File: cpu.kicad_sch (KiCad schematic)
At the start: 1 part

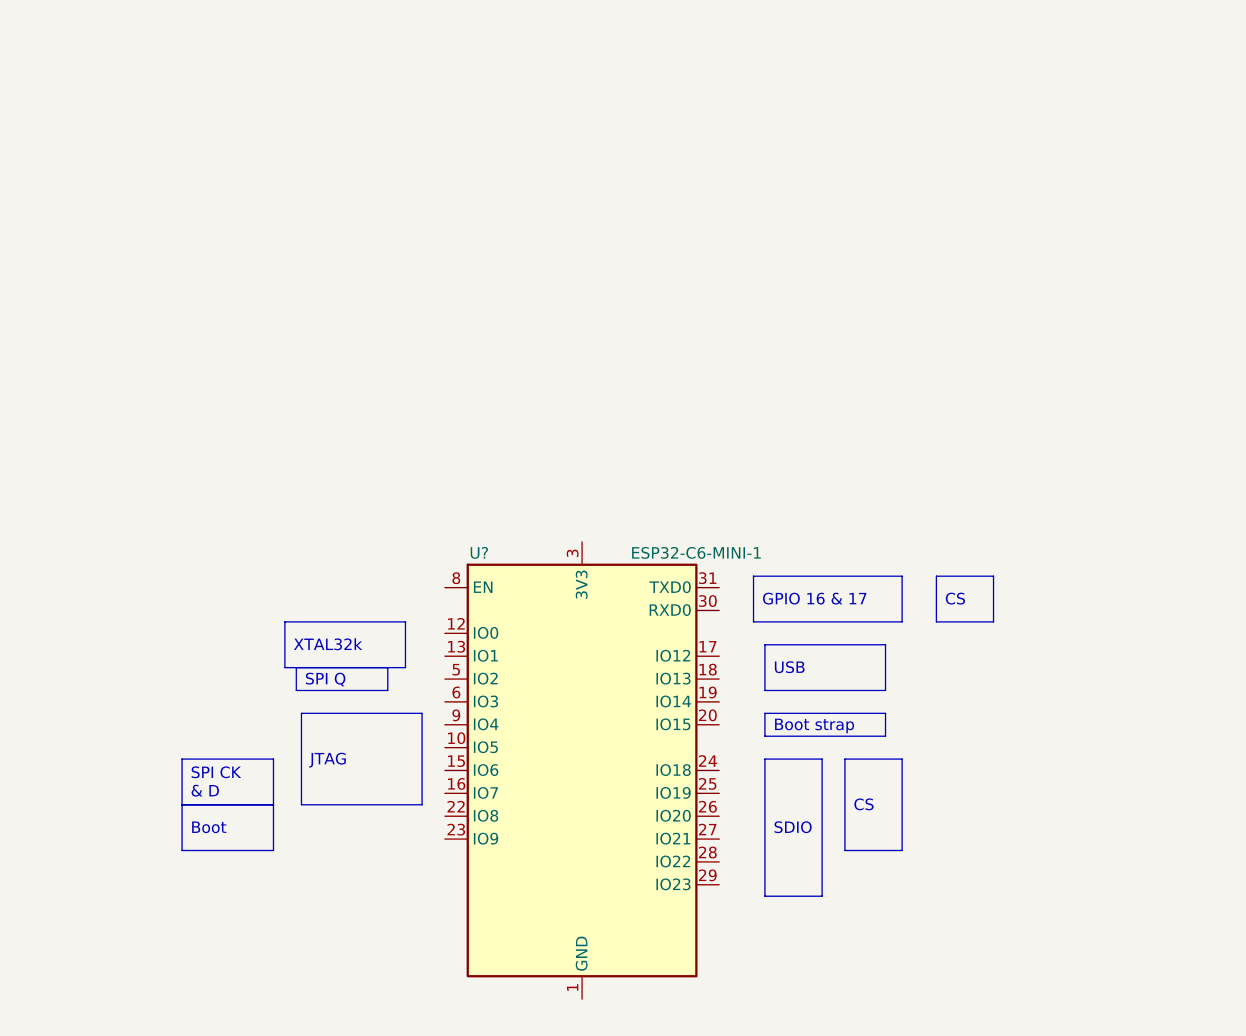
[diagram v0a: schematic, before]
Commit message: Schematic complete, maybe
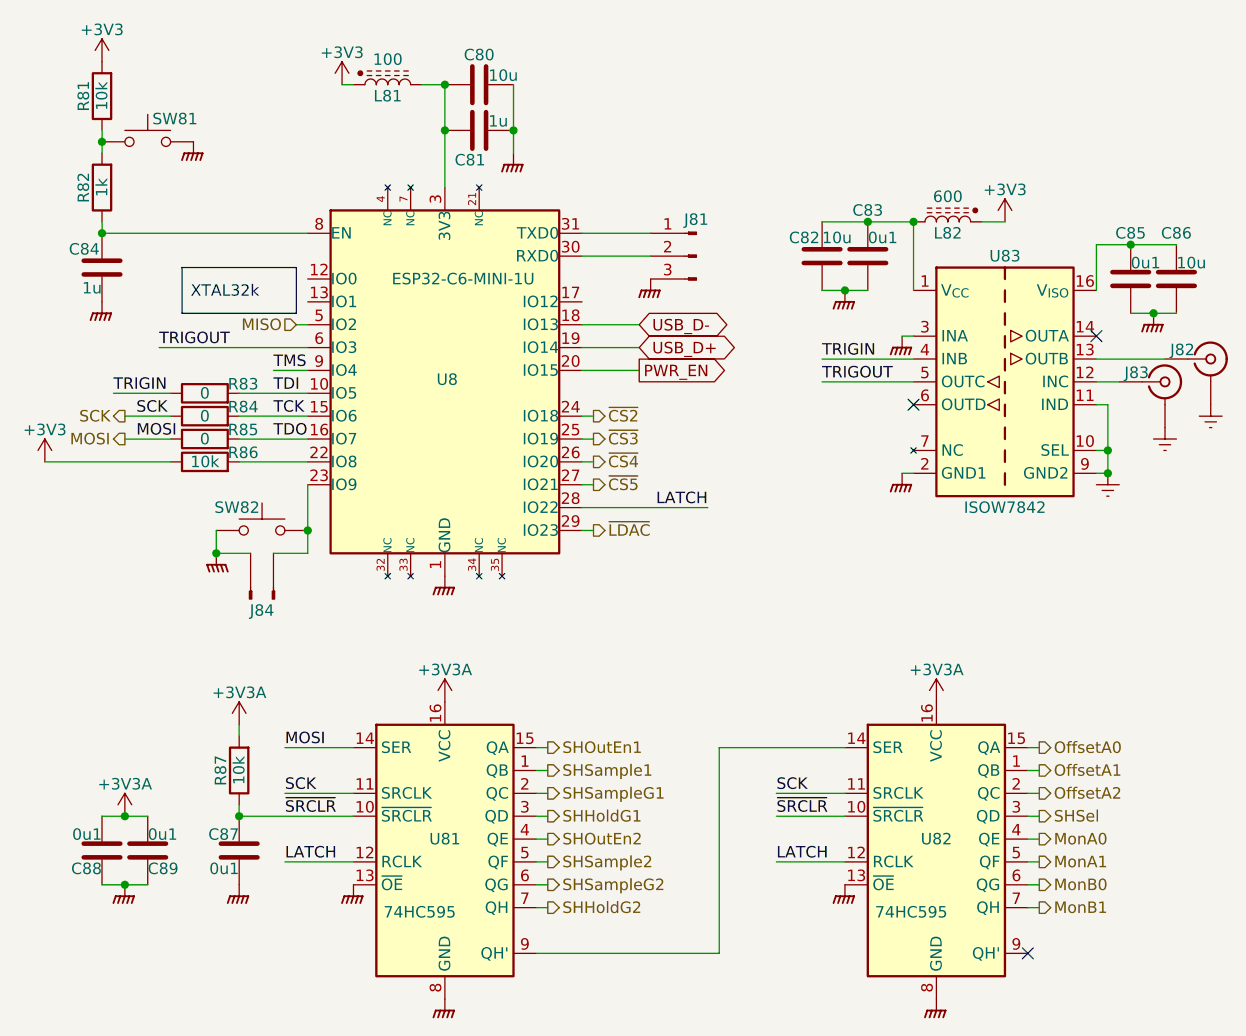
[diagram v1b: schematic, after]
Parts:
- removed U?: ESP32-C6-MINI-1, RF_Module:ESP32-C6-MINI-1, symbol RF_Module:ESP32-C6-MINI-1
- added C80, C82, C86: 10u, Capacitor_SMD:C_0603_1608Metric, symbol Device:C
- added C81, C84: 1u, Capacitor_SMD:C_0402_1005Metric, symbol Device:C
- added C83, C85, C87, C88, C89: 0u1, Capacitor_SMD:C_0402_1005Metric, symbol Device:C
- added J81: Conn_01x03_Pin, symbol Connector:Conn_01x03_Pin
- added J82, J83: Conn_Coaxial, symbol Connector:Conn_Coaxial
- added J84: Conn_01x02_Pin, symbol Connector:Conn_01x02_Pin
- added L81: 100, Inductor_SMD:L_0603_1608Metric, symbol Parts:L_Ferrite_Power
- added L82: 600, Inductor_SMD:L_0603_1608Metric, symbol Parts:L_Ferrite_Power
- added R81, R86, R87: 10k, Resistor_SMD:R_0402_1005Metric, symbol Device:R
- added R82: 1k, Resistor_SMD:R_0402_1005Metric, symbol Device:R
- added R83, R84, R85: 0, Resistor_SMD:R_0402_1005Metric, symbol Device:R
- added SW81, SW82: SW_Push, symbol Switch:SW_Push
- added U8: ESP32-C6-MINI-1U, RF_Module:ESP32-C6-MINI-1, symbol Parts:ESP32-C6-MINI-1U
- added U81, U82: 74HC595, Package_SO:SOIC-16_3.9x9.9mm_P1.27mm, symbol 74xx:74HC595
- added U83: ISOW7842, Package_SO:SOIC-16W_7.5x10.3mm_P1.27mm, symbol Parts:ISOW7842
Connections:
- new net: C82.1, C83.1, L82.2, U83.1 (V_{CC})
- new net: C80.1, C81.1, L81.2, U8.3 (3V3)
- new net: R81.1, R82.2, SW81.1
- new net: U81.9 (QH'), U82.14 (SER)
- new net: C84.1, R82.1, U8.8 (EN)
- new net: J83.1 (In), U83.12 (INC)
- new net: R86.2, U8.22 (IO8)
- new net: J82.1 (In), U83.13 (OUTB)
- new net: J81.1 (Pin_1), U8.31 (TXD0)
- new net: J81.2 (Pin_2), U8.30 (RXD0)
- new net: J84.1 (Pin_1), SW82.1, U8.23 (IO9)
- new net: C85.1, C86.1, U83.16 (V_{ISO})
- new net +3V3: L81.1, L82.1, R81.2, R86.1
- new net +3V3A: C88.1, C89.1, R87.2, U81.16 (VCC), U82.16 (VCC)
- new net Earth: J82.2 (Ext), J83.2 (Ext), U83.10 (SEL), U83.11 (IND), U83.15 (GND2), U83.9 (GND2)
- new net GND1: C80.2, C81.2, C82.2, C83.2, C84.2, C85.2, C86.2, C87.2, C88.2, C89.2, J81.3 (Pin_3), J84.2 (Pin_2), SW81.2, SW82.2, U8.1 (GND), U8.11 (GND), U8.14 (GND), U8.2 (GND), U8.36 (GND), U8.37 (GND), U8.38 (GND), U8.39 (GND), U8.40 (GND), U8.41 (GND), U8.42 (GND), U8.43 (GND), U8.44 (GND), U8.45 (GND), U8.46 (GND), U8.47 (GND), U8.48 (GND), U8.49 (GND), U8.50 (GND), U8.51 (GND), U8.52 (GND), U8.53 (GND), U81.13 (~{OE}), U81.8 (GND), U82.13 (~{OE}), U82.8 (GND), U83.2 (GND1), U83.3 (INA), U83.8 (GND1)
- new net LATCH: U8.28 (IO22), U81.12 (RCLK), U82.12 (RCLK)
- new net MISO: U8.5 (IO2)
- new net MOSI: R85.1, U81.14 (SER)
- new net MonA0: U82.4 (QE)
- new net MonA1: U82.5 (QF)
- new net MonB0: U82.6 (QG)
- new net MonB1: U82.7 (QH)
- new net OffsetA0: U82.15 (QA)
- new net OffsetA1: U82.1 (QB)
- new net OffsetA2: U82.2 (QC)
- new net PWR_EN: U8.20 (IO15)
- new net SCK: R84.1, U81.11 (SRCLK), U82.11 (SRCLK)
- new net SHHoldG1: U81.3 (QD)
- new net SHHoldG2: U81.7 (QH)
- new net SHOutEn1: U81.15 (QA)
- new net SHOutEn2: U81.4 (QE)
- new net SHSample1: U81.1 (QB)
- new net SHSample2: U81.5 (QF)
- new net SHSampleG1: U81.2 (QC)
- new net SHSampleG2: U81.6 (QG)
- new net SHSel: U82.3 (QD)
- new net TCK: R84.2, U8.15 (IO6)
- new net TDI: R83.2, U8.10 (IO5)
- new net TDO: R85.2, U8.16 (IO7)
- new net TMS: U8.9 (IO4)
- new net TRIGIN: R83.1, U83.4 (INB)
- new net TRIGOUT: U8.6 (IO3), U83.5 (OUTC)
- new net USB_D+: U8.19 (IO14)
- new net USB_D-: U8.18 (IO13)
- new net ~{CS2}: U8.24 (IO18)
- new net ~{CS3}: U8.25 (IO19)
- new net ~{CS4}: U8.26 (IO20)
- new net ~{CS5}: U8.27 (IO21)
- new net ~{LDAC}: U8.29 (IO23)
- new net ~{SRCLR}: C87.1, R87.1, U81.10 (~{SRCLR}), U82.10 (~{SRCLR})
- no-connect marks 0 -> 3

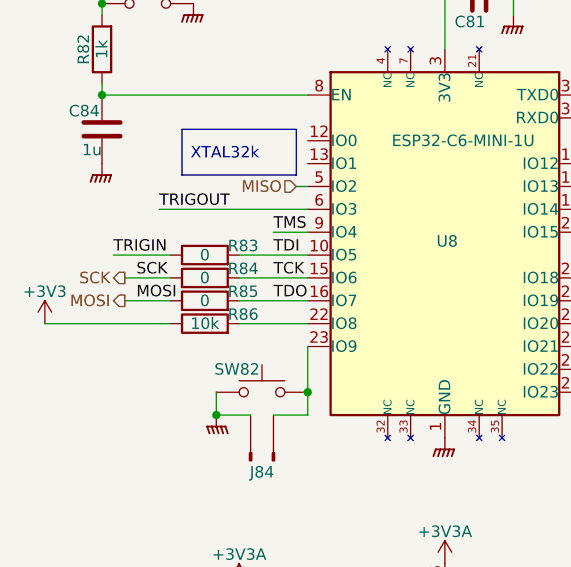
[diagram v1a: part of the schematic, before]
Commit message: Part selection
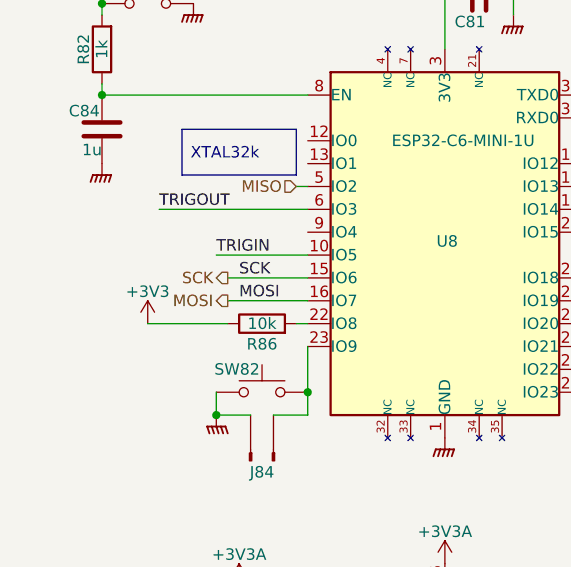
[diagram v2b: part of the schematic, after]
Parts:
- removed R83, R84, R85: 0, Resistor_SMD:R_0402_1005Metric, symbol Device:R
- J81, J82, J83, J84: now left out of the parts list
- R81, R86, R87: LCSC (none) -> C25744
- R82: LCSC (none) -> C11702
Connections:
- net TCK is gone; now on net SCK: U8.15 (IO6)
- net TDI is gone; now on net TRIGIN: U8.10 (IO5)
- net TDO is gone; now on net MOSI: U8.16 (IO7)
- net TMS: no longer names the net of U8.9 (IO4)
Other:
- moved on the sheet: R86
